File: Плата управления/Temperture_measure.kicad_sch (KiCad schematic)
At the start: 14 parts, among them U8 LMV324

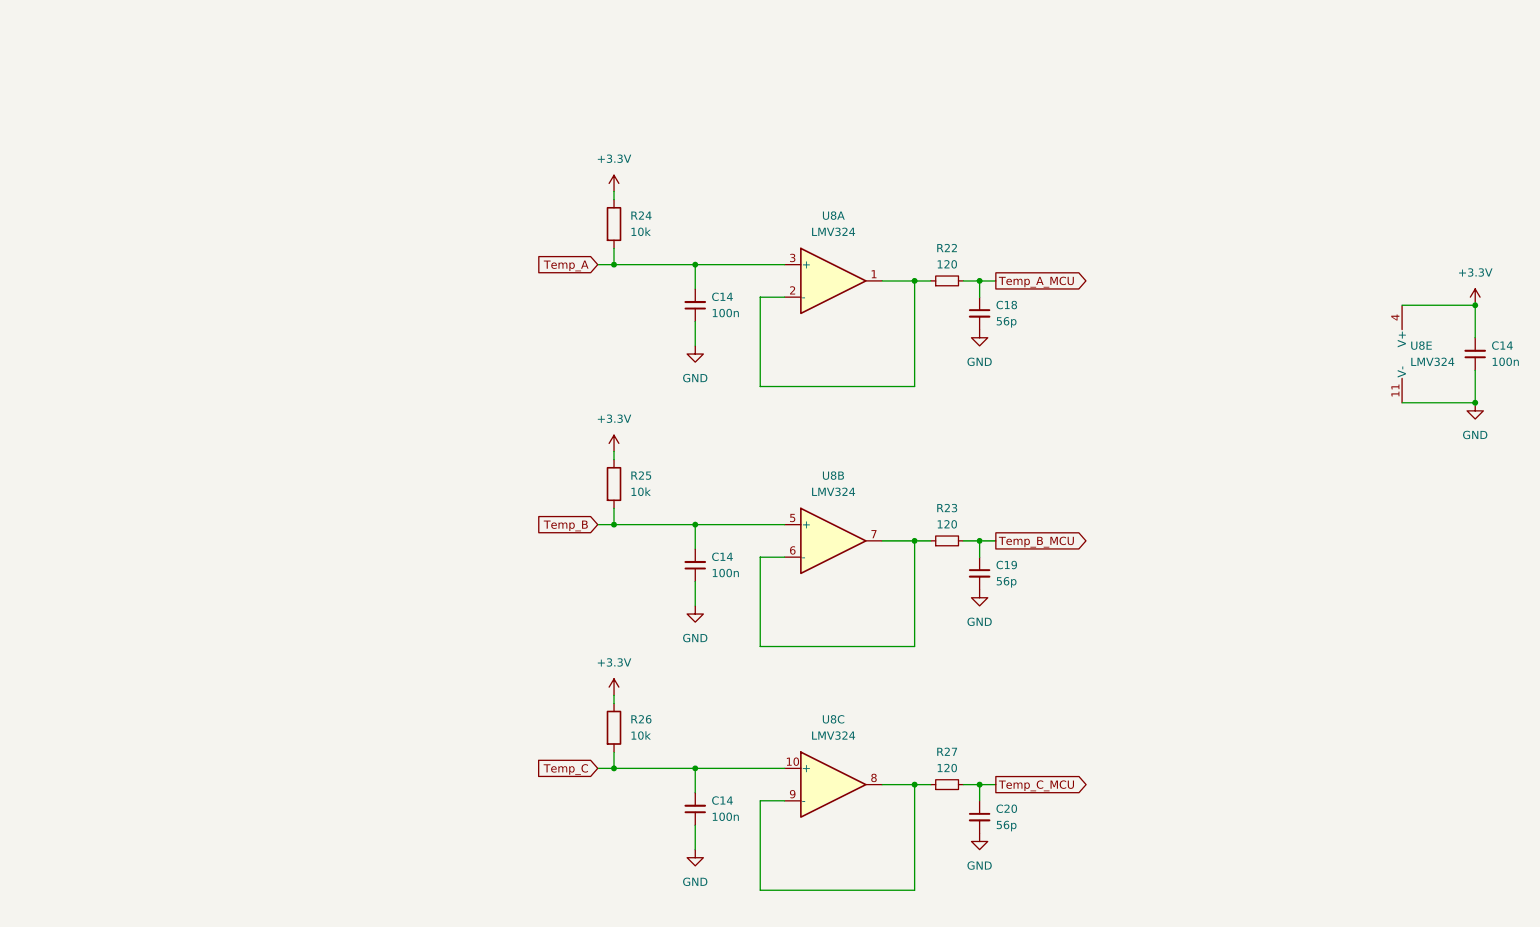
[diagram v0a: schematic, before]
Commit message: Привел в порядок схему
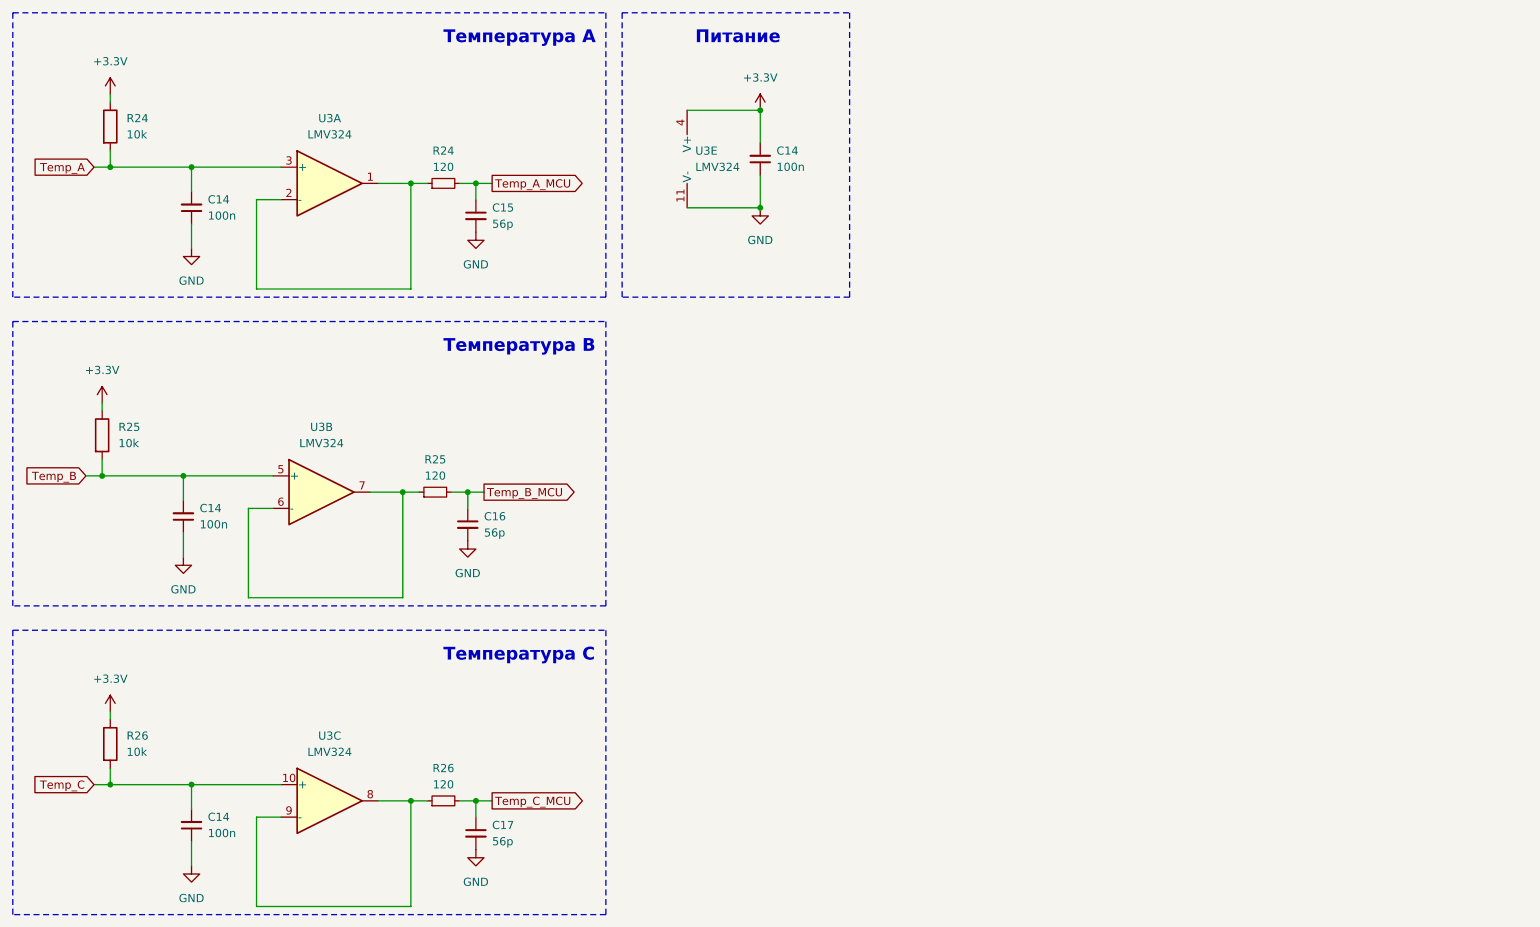
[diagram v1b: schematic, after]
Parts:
- renumbered C18 to C15, C19 to C16, C20 to C17, R22 to R24, R23 to R25, R27 to R26, U8 to U3
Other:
- note added: "Питание"
- note added: "Температура А"
- note added: "Температура В"
- note added: "Температура С"
- moved on the sheet: C14, C15, C16, C17, R24, R25, R26, U3A, U3B, U3C, U3E
